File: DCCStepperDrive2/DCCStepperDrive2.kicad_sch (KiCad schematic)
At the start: 33 parts, among them J1 12v, J2 CBUS, J3 5V select, J4 DCC, J5 Grove 2mm, J6 I2C, J7 Sensor, J8 Motor, J9 Mode Select, Q1 DMG2305UX-7, SW1 SW_Push, U1 AMS1117-3.3, U2 AMS1117-5.0, U3 6N137, U4 Pico, U5 CAT24C256

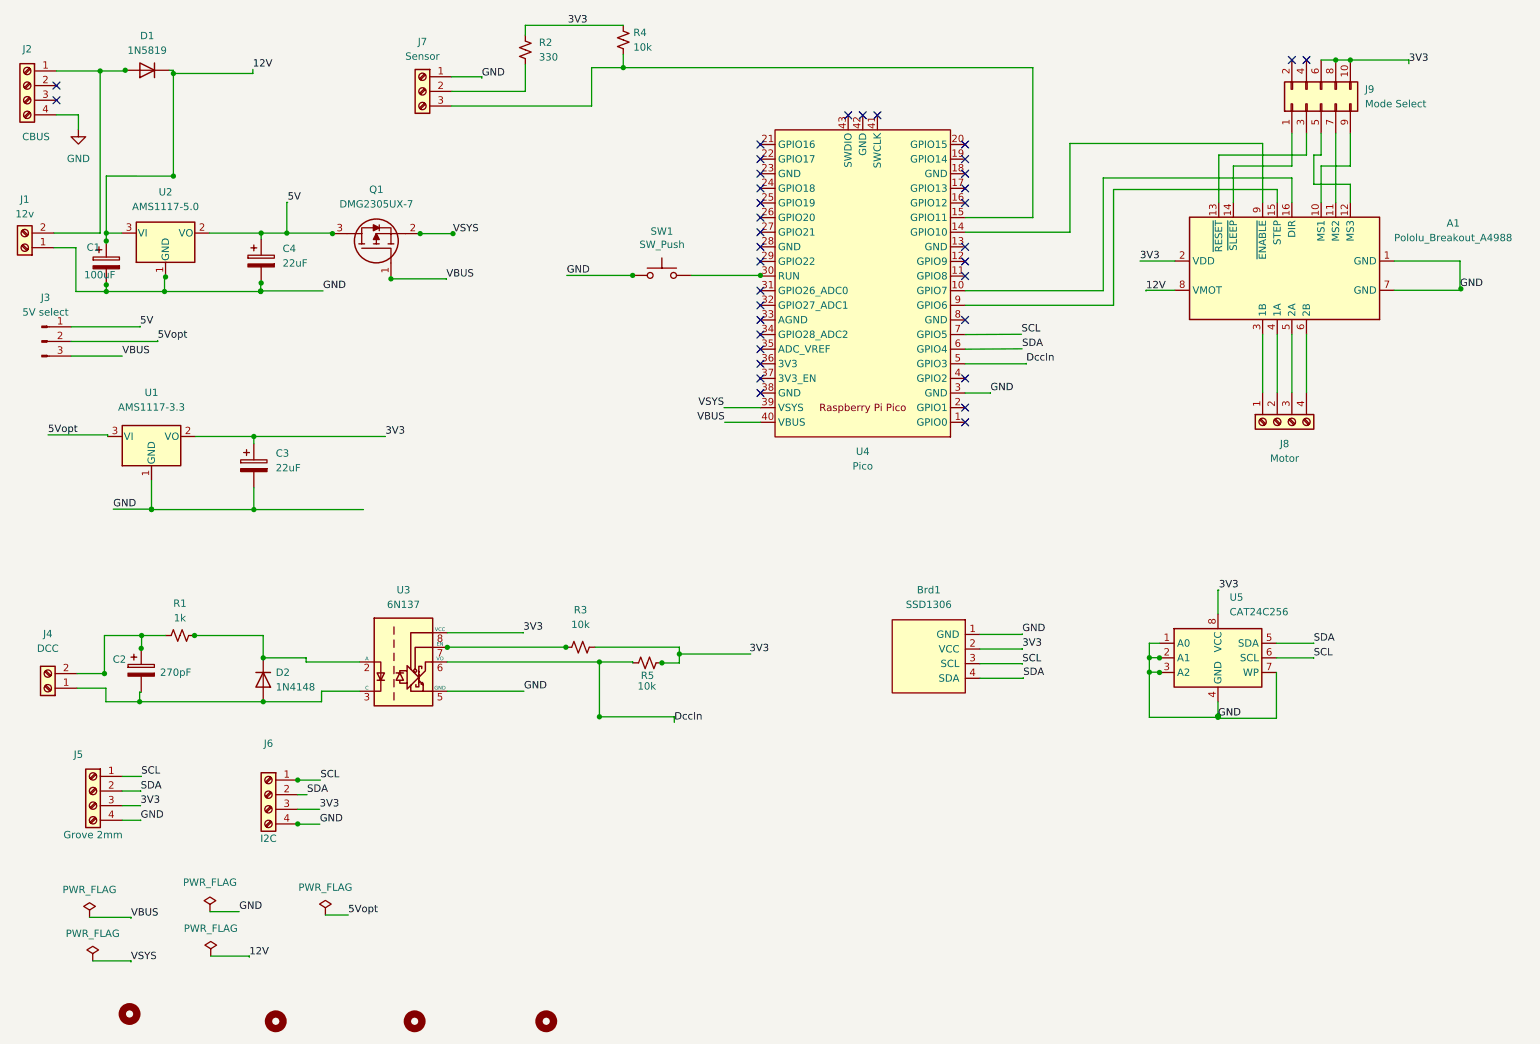
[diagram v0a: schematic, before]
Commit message: 09/09/25 09:18 Arrakis.local
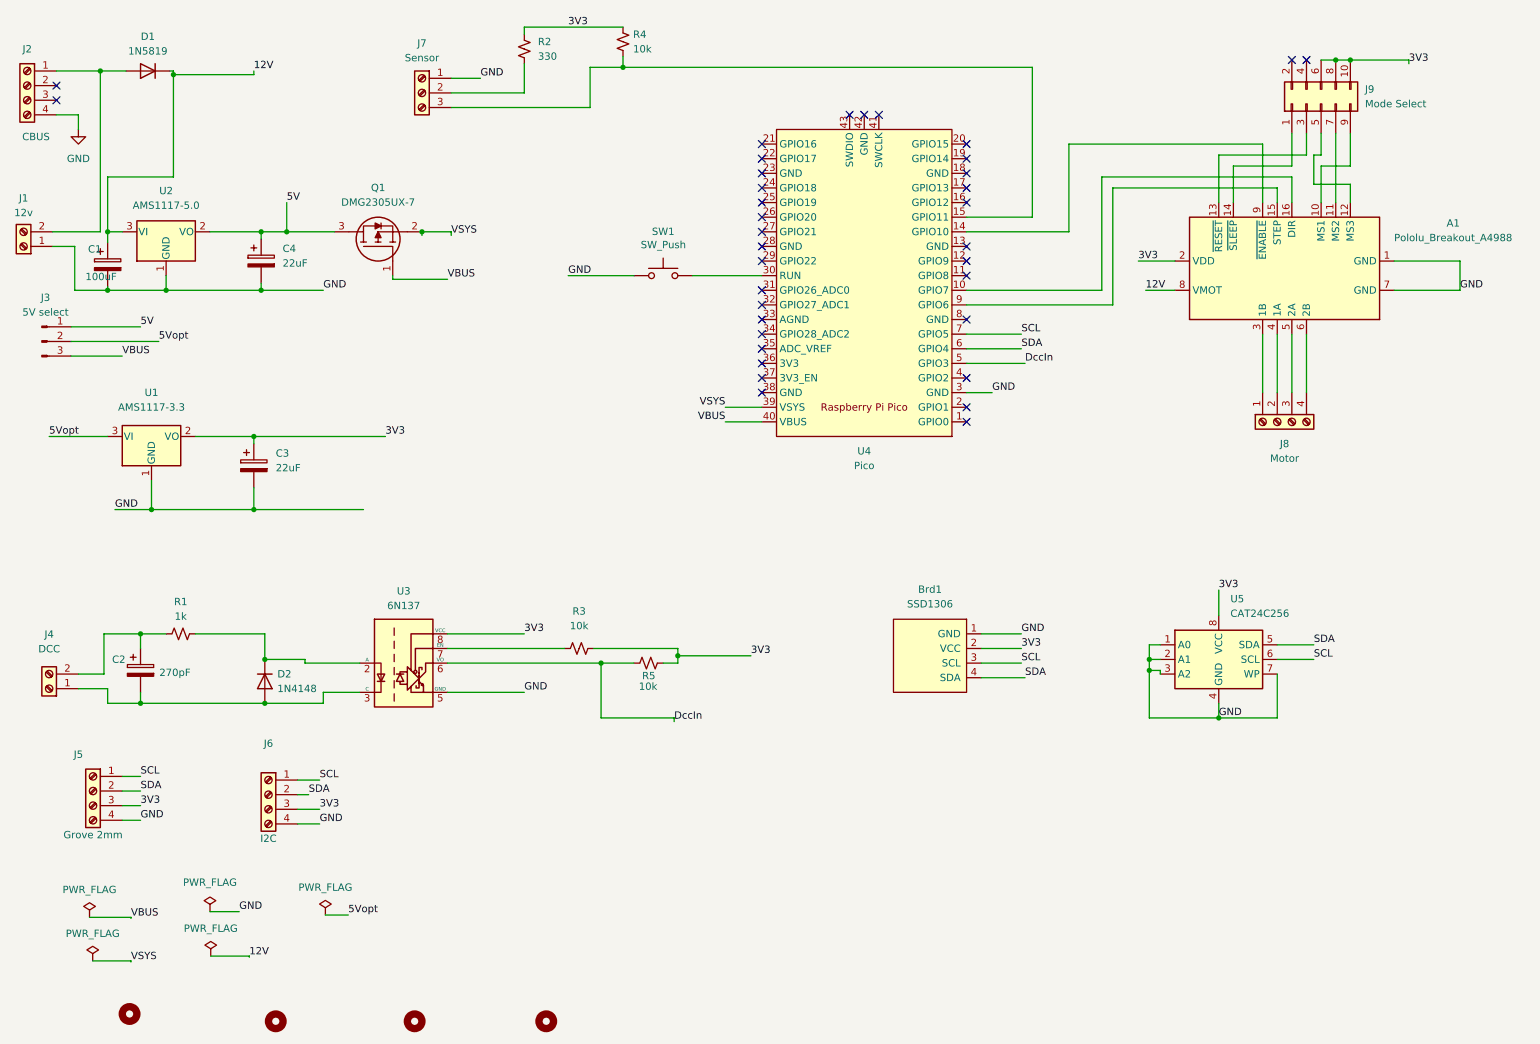
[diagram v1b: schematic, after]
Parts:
- J5, J6: footprint OPL_Connector:HW4-2.0 -> OPL_Kicad_Library:HW4-2.0
- U4: footprint MCU_RaspberryPi_and_Boards:RP2040Pico -> Kicad-RP-Pico:RPi_Pico_SMD_TH

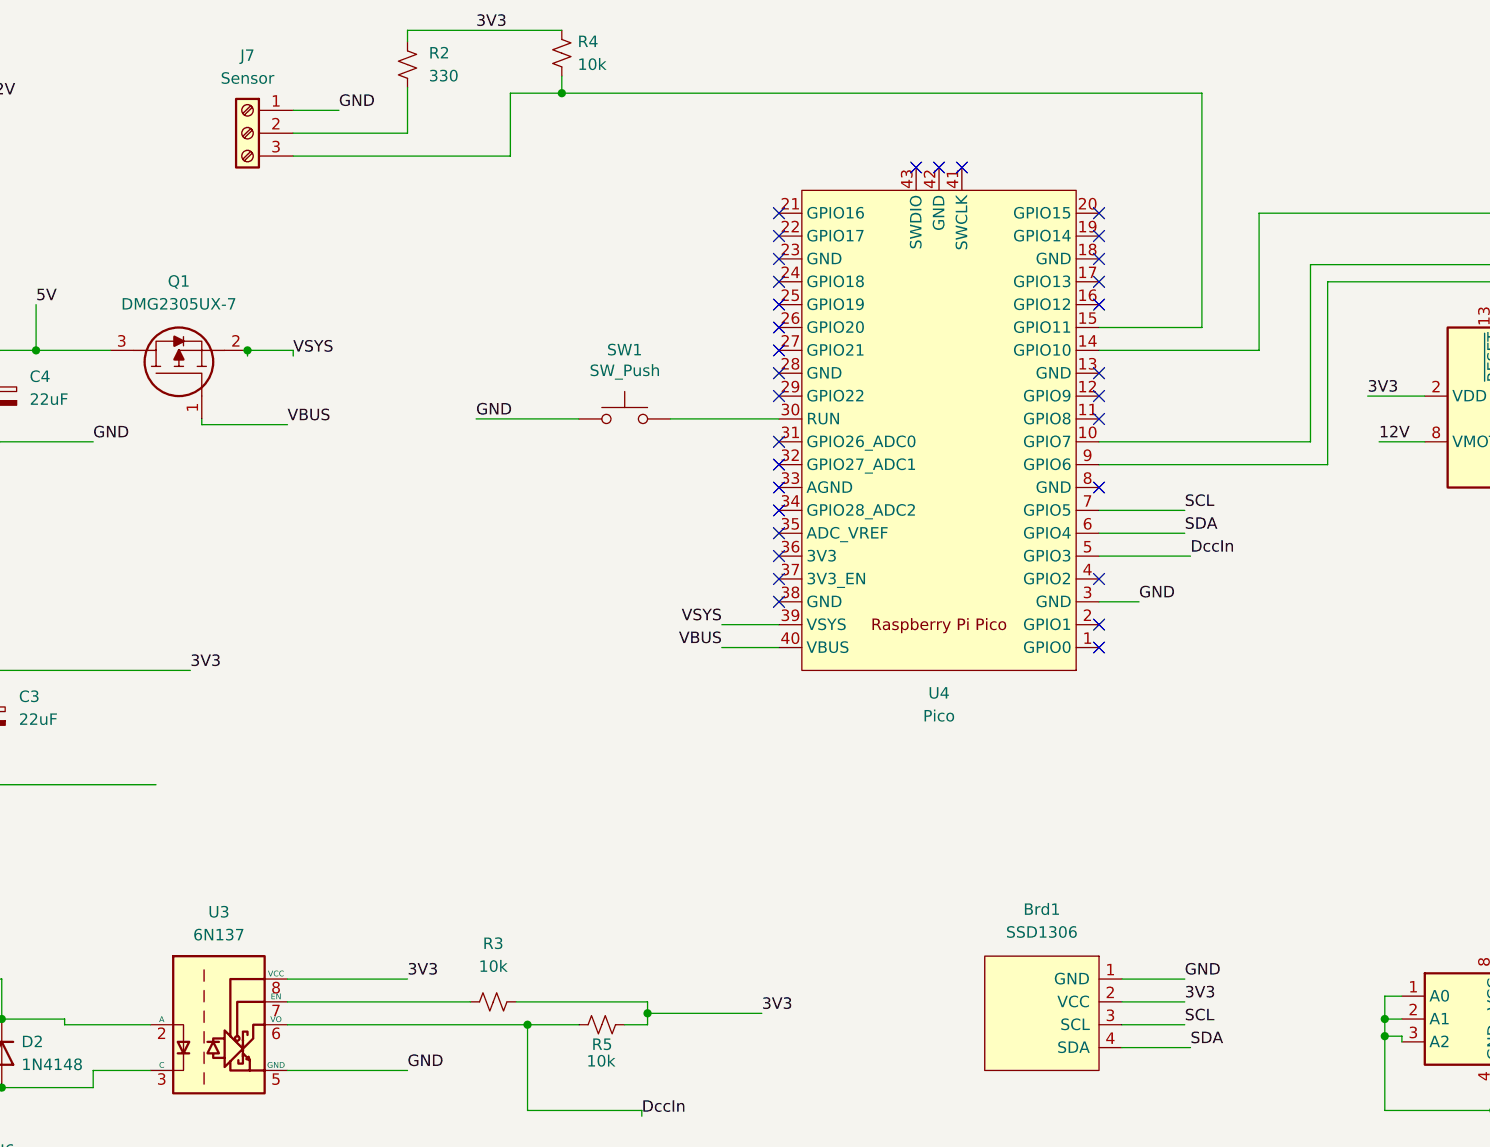
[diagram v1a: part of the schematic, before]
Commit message: 09/09/25 10:15 Titan.local
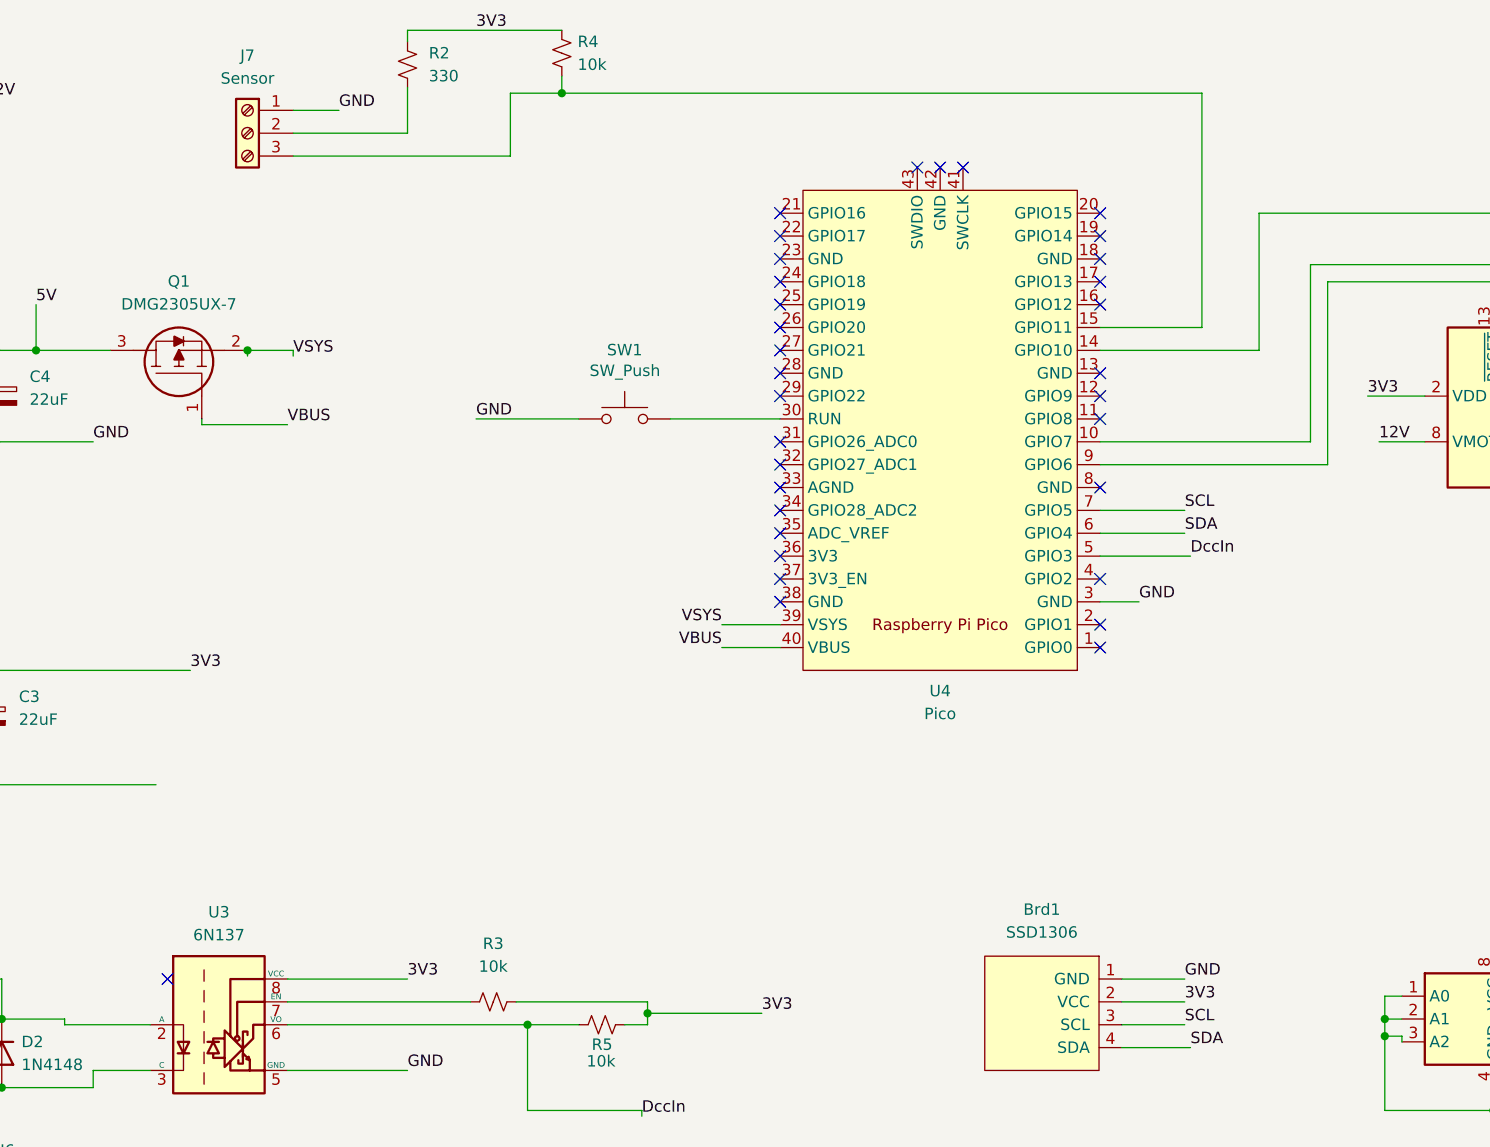
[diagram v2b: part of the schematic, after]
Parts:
- removed U4: Pico, Kicad-RP-Pico:RPi_Pico_SMD_TH, symbol MCU_RaspberryPi_and_Boards:Pico
- added U4: Pico, Kicad-RP-Pico:RPi_Pico_SMD_TH, symbol Kicad-RP-Pico:Pico
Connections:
- net DccIn: now also U4.5 (GPIO3)
- net GND: now also U4.3 (GND)
- net SCL: now also U4.7 (GPIO5)
- net SDA: now also U4.6 (GPIO4)
- net VBUS: now also U4.40 (VBUS)
- net VSYS: now also U4.39 (VSYS)
- net at A1.15 (STEP): now also U4.9 (GPIO6)
- net at A1.16 (DIR): now also U4.10 (GPIO7)
- net at A1.9 (~{ENABLE}): now also U4.14 (GPIO10)
- net at J7.3 (Pin_3), R4.1: now also U4.15 (GPIO11)
- net at SW1.2: now also U4.30 (RUN)
- no-connect marks 36 -> 37

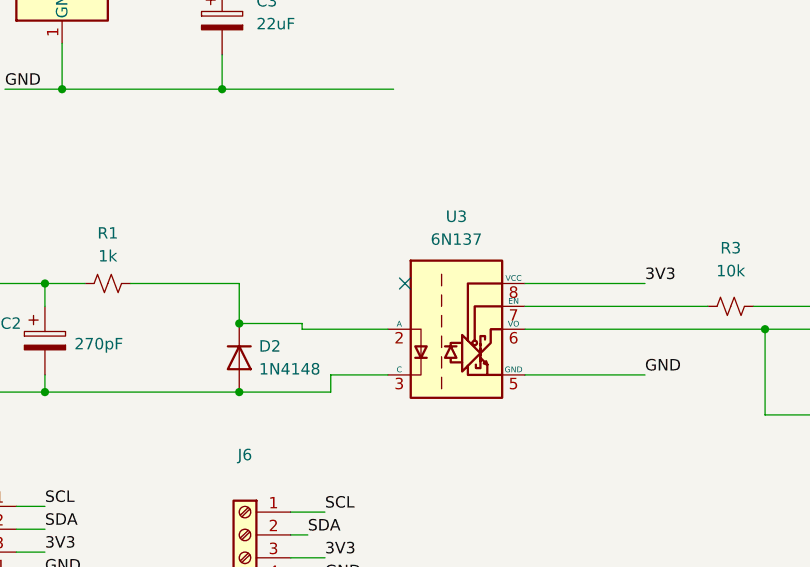
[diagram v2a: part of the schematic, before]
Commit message: 10/09/25 13:02 Titan.local
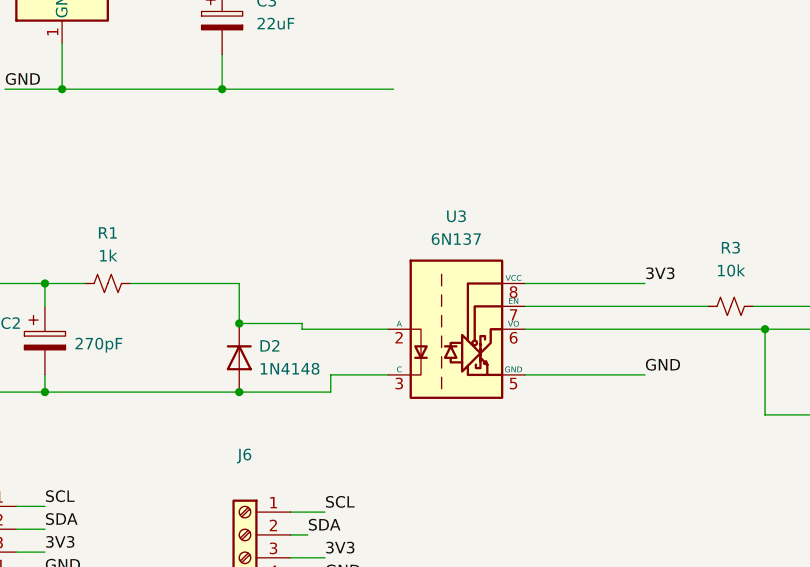
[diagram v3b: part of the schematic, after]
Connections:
- no-connect marks 37 -> 36
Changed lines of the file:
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@@
   (no_connect (at 145.542 39.37))
   (no_connect (at 181.102 44.45))
-  (no_connect (at 77.47 121.92))
   (no_connect (at 145.542 74.93))
   (no_connect (at 181.102 59.69))
